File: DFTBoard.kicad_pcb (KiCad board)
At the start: 2 copper layers, 271 parts, among them CON1 AVR-JTAG-10, CON2 AVR-JTAG-10, IC1 WM8758B, IC2 IS31FL3199, IC3 CyUSB30xx-BZX, J1 JACK_TRS_6PINS, J2 JACK_TRS_6PINS, J3 JACK_TRS_6PINS, J4 JACK_TRS_6PINS, J5 MICRO_HDMI, J6 GSB3211311WEU, J7 48258-0001, Q1 IRLML2502, Q2 IRLML2502, Q3 IRLML2502, Q4 IRLML2502, Q5 IRLML2502, U1 xc7a50tftg256, U10 MAX3421, U11 GTL2002, U12 NC7WZ07P6X, U13 NC7SZ125M5X, U14 ADP198ACPZ-R7, U2 24FC128, U3 N25Q128A, U5 SC189 - 3.3V, U6 SC189 - 1.0V, U7 SC189 - 1.2V, U8 SC189 - 1.8V, U9 VL53L0X, X1 KC5032A, Y1 19.2MHz, Y2 12MHz

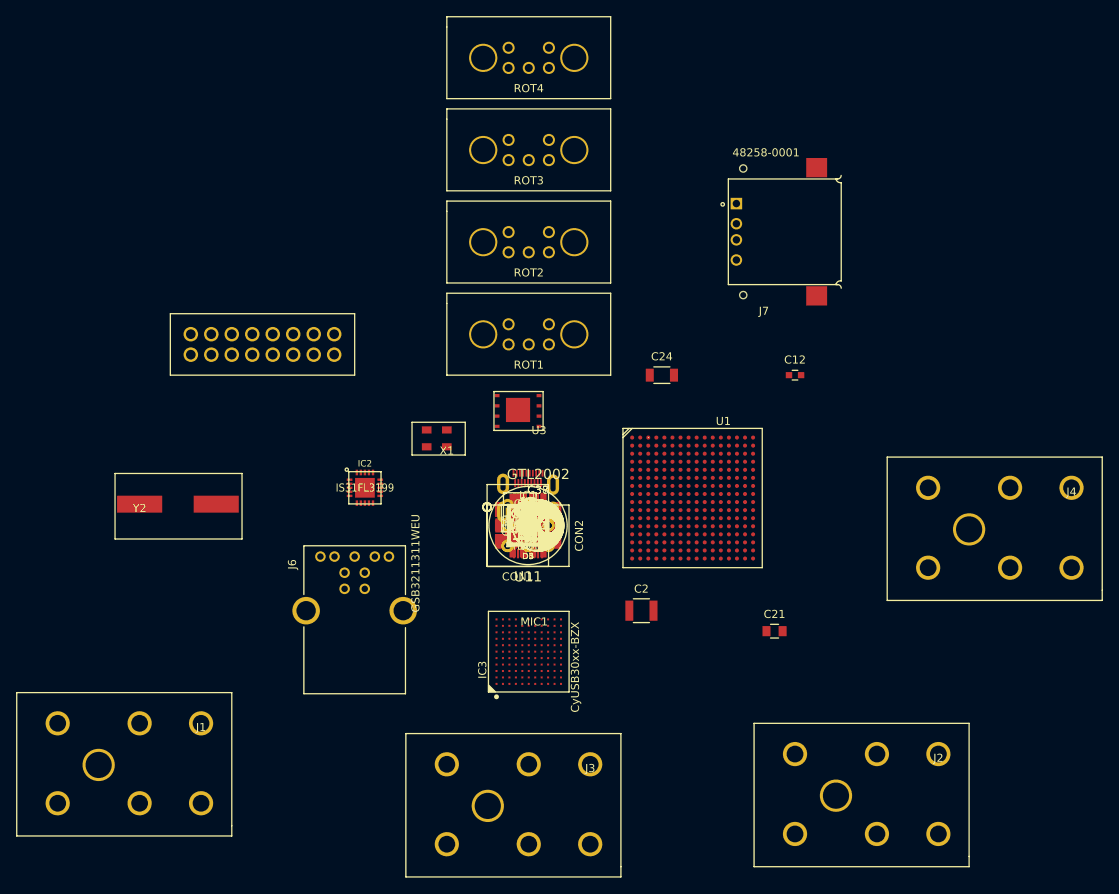
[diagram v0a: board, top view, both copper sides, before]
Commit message: a few small changes
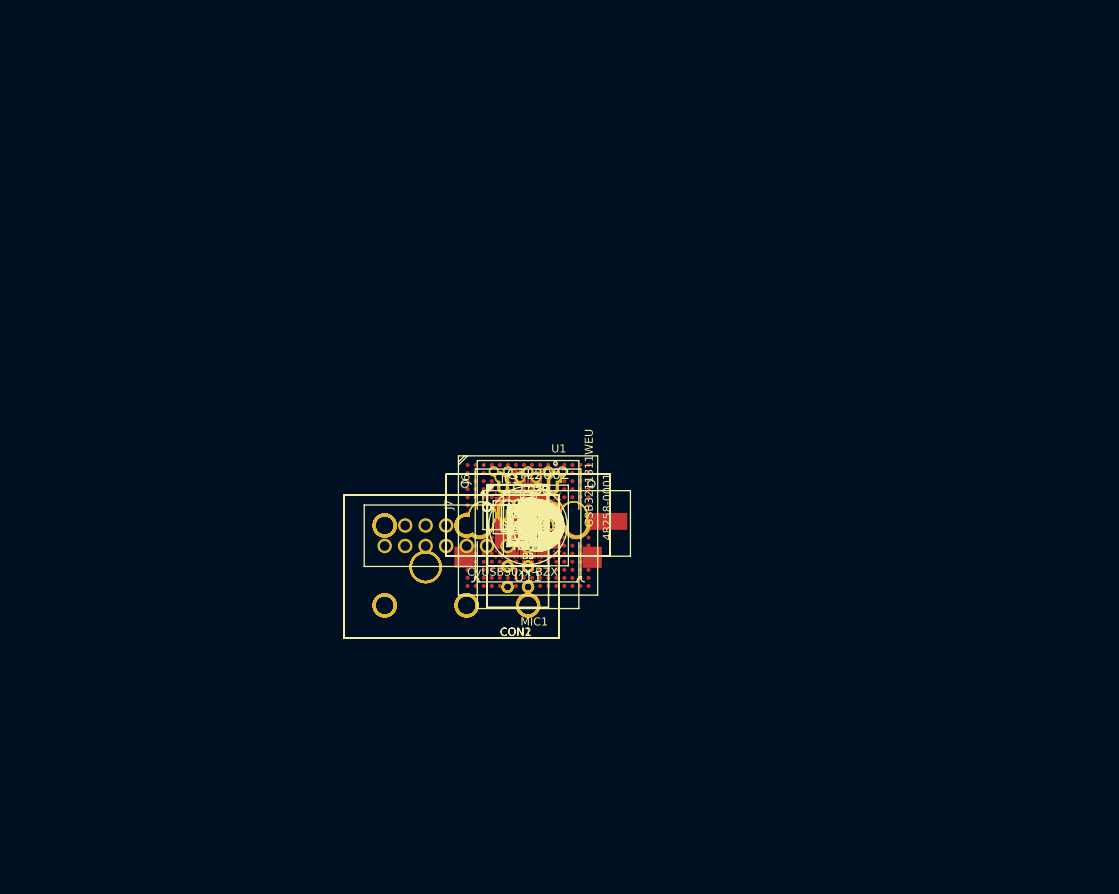
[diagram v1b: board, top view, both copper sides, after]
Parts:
- moved J4 67.6 mm to (148.5, 105.0)
- moved J2 58.3 mm to (148.5, 105.0)
- moved ROT4 56.7 mm to (148.5, 105.0)
- moved J7 48.4 mm to (148.5, 105.0), turned to 0 degrees
- moved Y2 48.2 mm to (148.5, 105.0)
- moved J1 47.4 mm to (148.5, 105.0)
- moved ROT3 45.3 mm to (148.5, 105.0)
- moved C12 38.0 mm to (148.5, 105.0)
- moved ROT2 33.9 mm to (148.5, 105.0)
- moved DS1 33.8 mm to (148.5, 105.0)
- moved C21 33.3 mm to (148.5, 105.0)
- moved J3 30.6 mm to (148.5, 105.0)
- moved C24 25.0 mm to (148.5, 105.0)
- moved J6 24.0 mm to (148.5, 105.0)
- moved ROT1 22.5 mm to (148.5, 105.0)
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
